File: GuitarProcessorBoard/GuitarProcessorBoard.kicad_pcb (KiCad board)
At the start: 4 copper layers, 134 parts, among them J301 SWD Header, J302 PWR, J303 TAP, J304 MODE, J305 BYP, J306 EXP, J307 ScopeGroundLoop, SW301 RST, SW302 BOOT, U201 TLV320AIC3204, U202 TL074, U301 STM32H7B0VBT6, U302 TPS63070, U303 SSD1306_OLED_128x64, U304 74HC595, Y301 32MHz, Y302 32.768kHZ

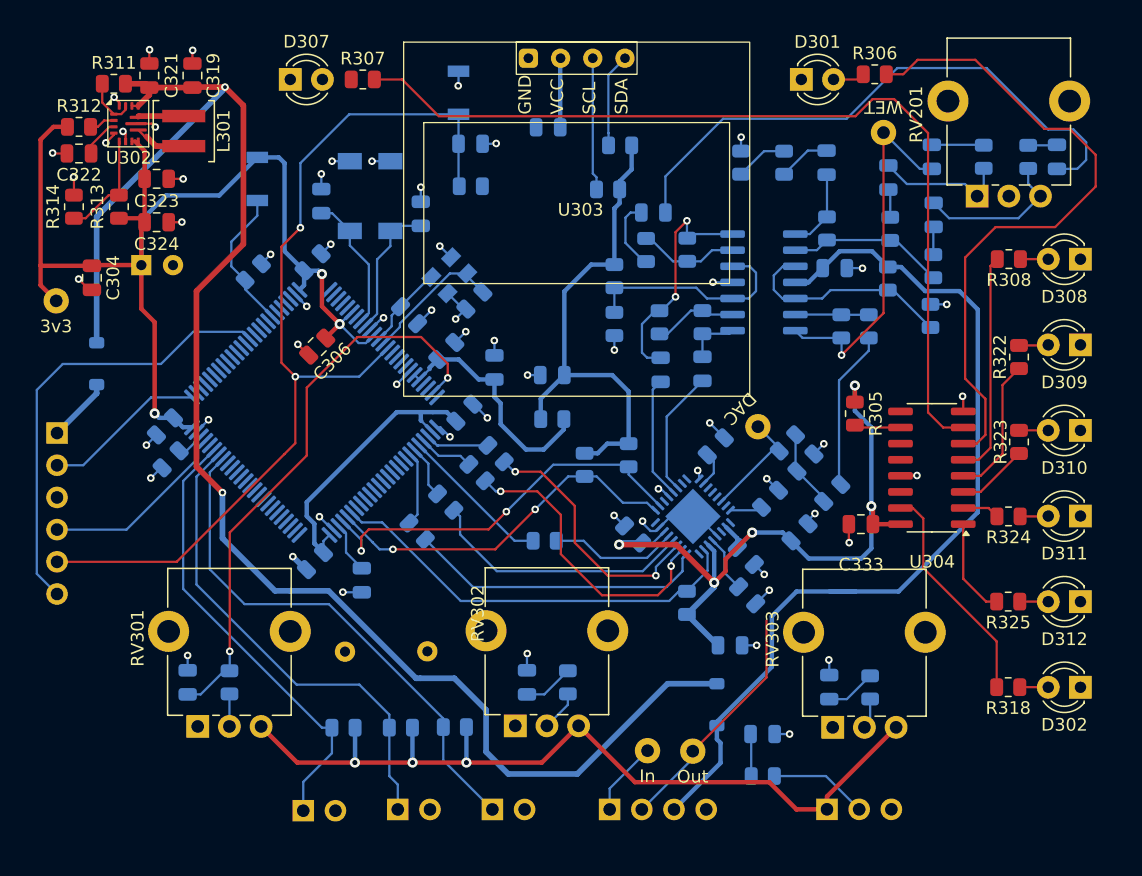
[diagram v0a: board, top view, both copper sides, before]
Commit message: routed & DRC passing
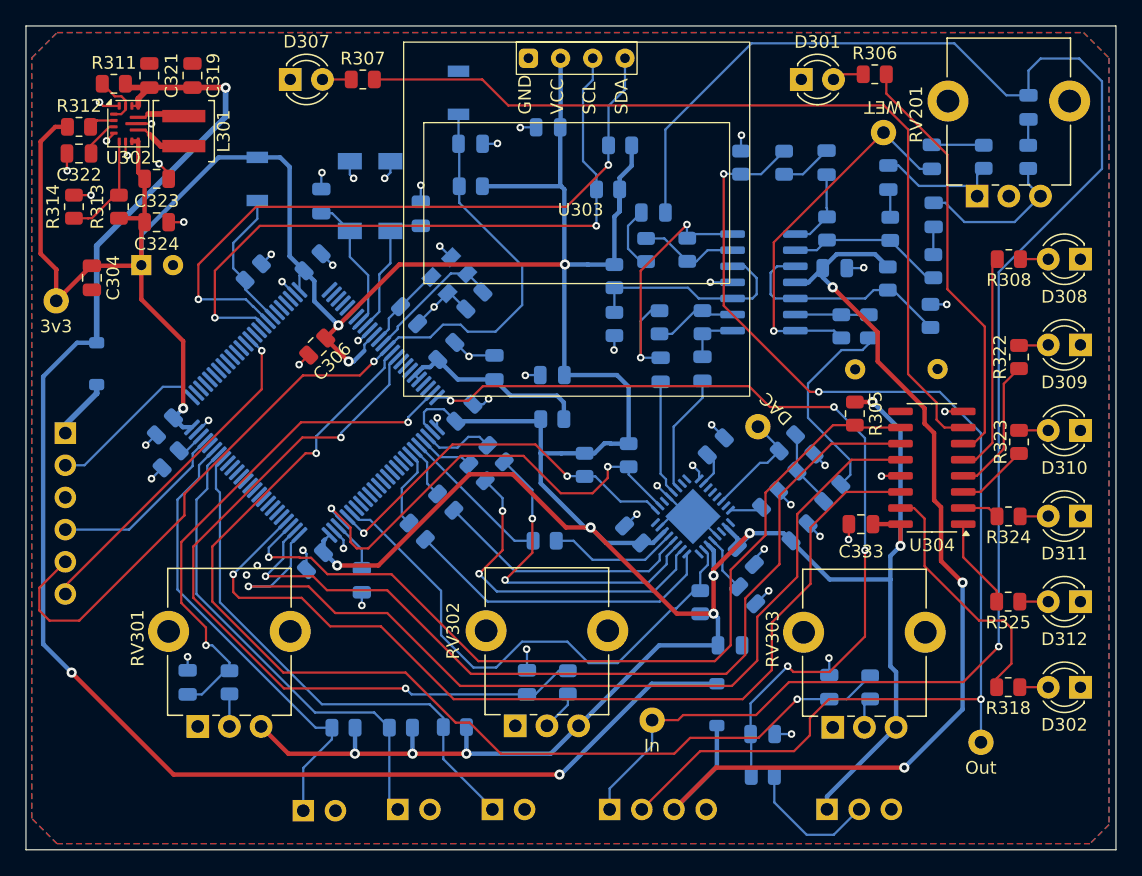
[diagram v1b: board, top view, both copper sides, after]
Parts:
- moved J307 46.0 mm to (-110.5, 58.0)
- moved TP302 22.8 mm to (-103.6, 87.5)
- moved C207 4.51 mm to (-99.8, 37.4), turned to -90 degrees
- moved TP301 2.44 mm to (-129.6, 85.8)
- moved R201 1.05 mm to (-125.8, 76.5)
- moved J301 0.65 mm to (-175.8, 63.1)
- turned TP202 to -45 degrees
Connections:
- U301 pad 1: LED_SCK -> unconnected-(U301-PE2-Pad1)
- U301 pad 3: LED_LATCH -> unconnected-(U301-PE4-Pad3)
- U301 pad 4: LED_NRST -> unconnected-(U301-PE5-Pad4)
- U301 pad 5: LED_DATA -> unconnected-(U301-PE6-Pad5)
- U301 pad 51: unconnected-(U301-PB12-Pad51) -> LED_LATCH
- U301 pad 52: unconnected-(U301-PB13-Pad52) -> LED_SCK
- U301 pad 53: unconnected-(U301-PB14-Pad53) -> LED_NRST
- U301 pad 54: unconnected-(U301-PB15-Pad54) -> LED_DATA
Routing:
- net FX_IN: track 51.9 -> 134.8 mm, vias 0 -> 1
- net ADC_C: track 3.99 -> 85.4 mm, vias 0 -> 2
- net LED_DATA: track 0.00 -> 75.0 mm, vias 0 -> 1
- net +3.3V: track 287.8 -> 362.8 mm, vias 11 -> 14
- net LED_LATCH: track 0.00 -> 73.8 mm, vias 0 -> 1
- net FX_OUT: track 23.1 -> 95.9 mm, vias 0 -> 3
- net LED_SCK: track 0.00 -> 71.2 mm, vias 0 -> 1
- net LED_NRST: track 3.68 -> 69.4 mm, vias 0 -> 1
- net ADC_EXP: track 3.34 -> 69.0 mm, vias 0 -> 4
- net ADC_B: track 4.00 -> 60.9 mm, vias 0 -> 2
- net DISP_SDA: track 7.42 -> 53.5 mm, vias 0 -> 2
- net DISP_SCL: track 10.9 -> 53.4 mm, vias 0 -> 2
- net /MCU/LED_TEMPO: track 51.9 -> 32.7 mm
- net SWO: track 35.7 -> 26.3 mm, vias 0 -> 1
- net +9V: track 73.7 -> 82.1 mm, vias 0 -> 3
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- added copper zone on B.Cu, net GND
- added copper zone on F.Cu, net GND
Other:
- board outline added: 86 x 65 mm
